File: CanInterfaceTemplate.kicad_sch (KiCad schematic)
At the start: 7 parts, among them U1 MCP2515-xSO, U2 MCP2551-I-P, Y1 16M

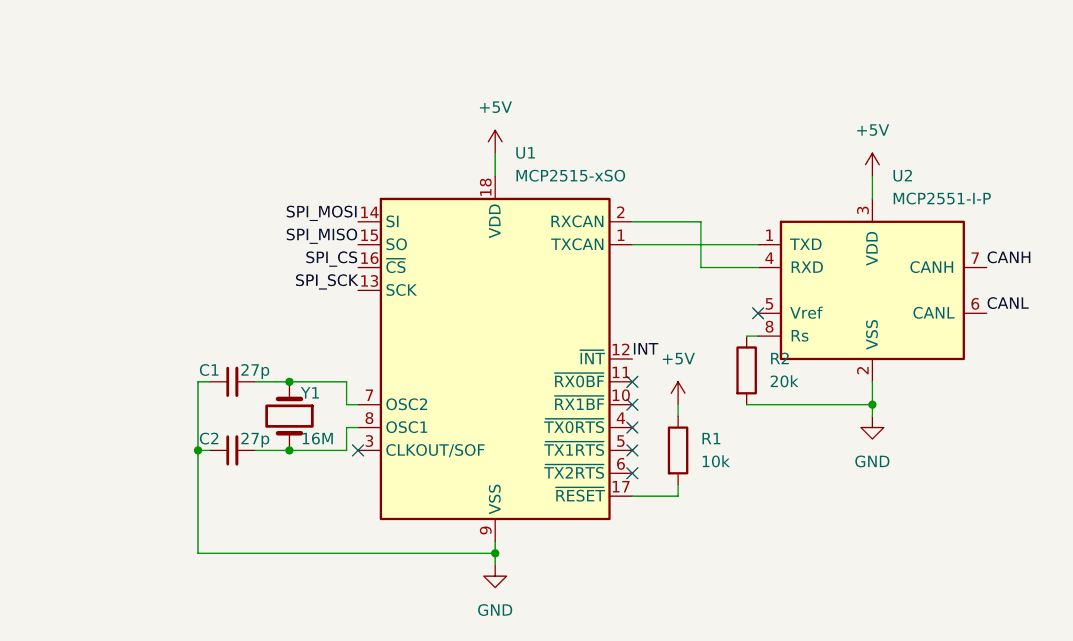
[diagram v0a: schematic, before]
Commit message: Add updated KiCAD templates
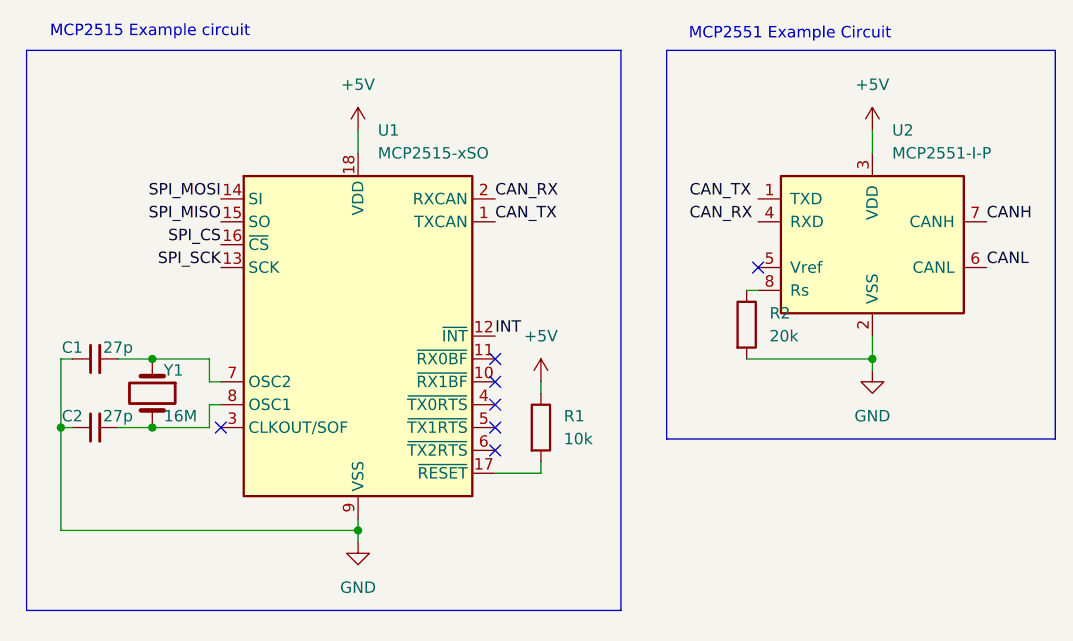
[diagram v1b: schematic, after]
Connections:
- net at U2.1 (TXD): no longer U1.1 (TXCAN)
- net at U2.4 (RXD): no longer U1.2 (RXCAN)
- new net CAN_RX: U1.2 (RXCAN)
- new net CAN_TX: U1.1 (TXCAN)
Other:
- note added: "MCP2515 Example circuit"
- note added: "MCP2551 Example Circuit"
- moved on the sheet: C1, C2, R1, R2, U1, U2, Y1
